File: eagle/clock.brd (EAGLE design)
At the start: 100 x 80 mm, 0 parts

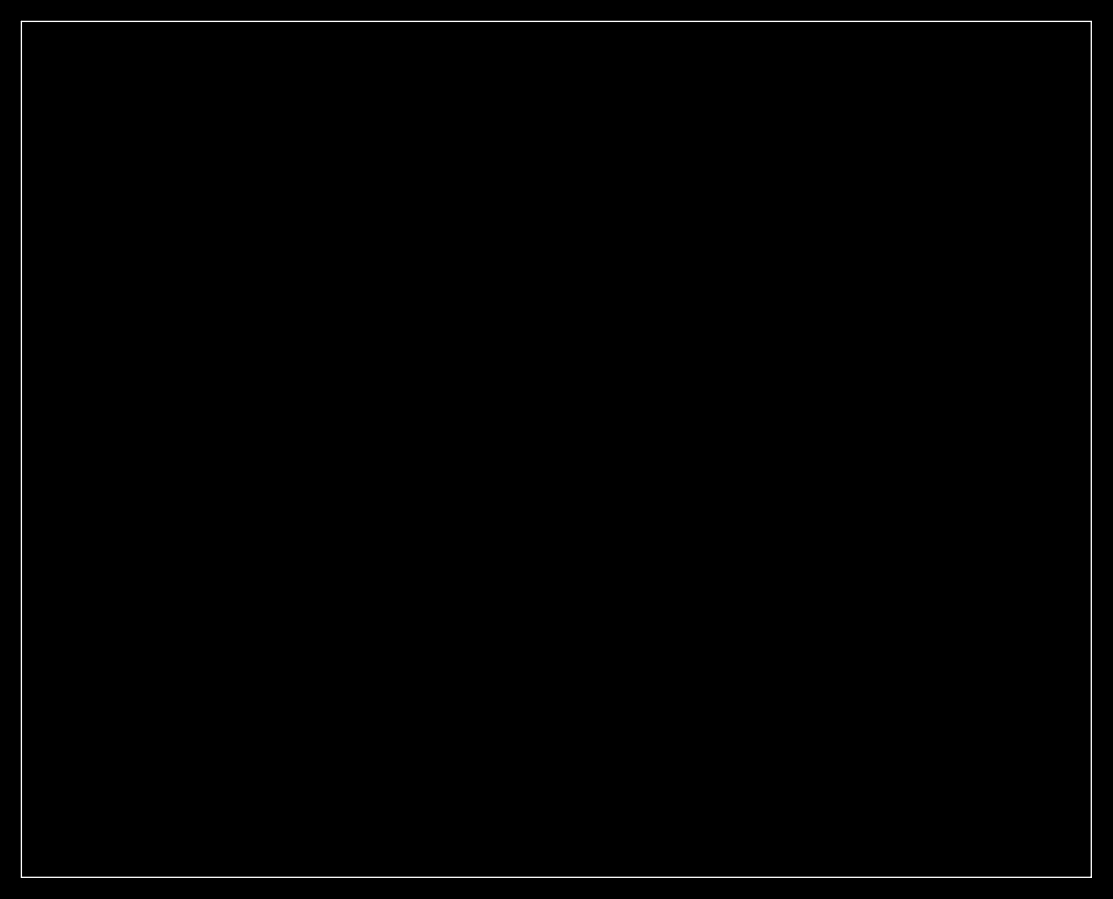
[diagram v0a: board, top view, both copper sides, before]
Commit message: .
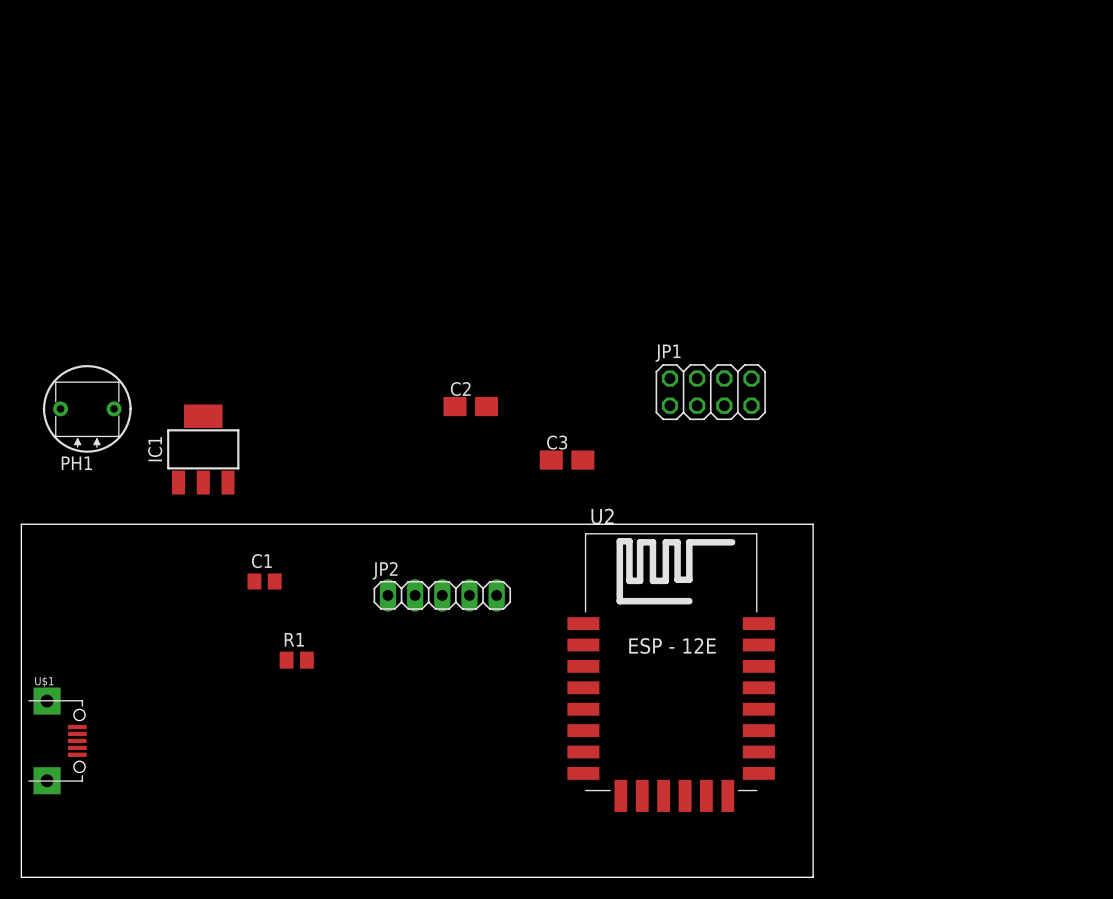
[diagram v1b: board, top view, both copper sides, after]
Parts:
- added C1: (no value), rcl:C0805
- added C2: 10mF, rcl:A/3216-18W
- added C3: 100mF, rcl:A/3216-18W
- added IC1: LM1117MPX-3.3, lm1117:SOT223
- added JP1: (no value), pinhead:2X04
- added JP2: (no value), pinhead:1X05
- added PH1: D1160_12, photo-elements:D11XX
- added R1: (no value), rcl:M0805
- added U$1: MICRO-USB, microusb:MICRO-USB
- added U2: (no value), esp8266modules:ESP12E-SMD
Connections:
- new net +3V3: C3.+, IC1.2, IC1.TAB, U2.VCC
- new net +5V: C2.+, IC1.3, U$1.1
- new net GND: C2.-, C3.-, IC1.1, U$1.5, U$1.GND1, U$1.GND2, U2.GND
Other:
- board size 100 x 80 mm -> 74 x 33 mm
